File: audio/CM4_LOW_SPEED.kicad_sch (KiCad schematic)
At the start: 8 parts, among them J4 THD-02-R, U5 TPD4EUSB30, U6 TPD4EUSB30, U7 MagJack-A70-112-331N126

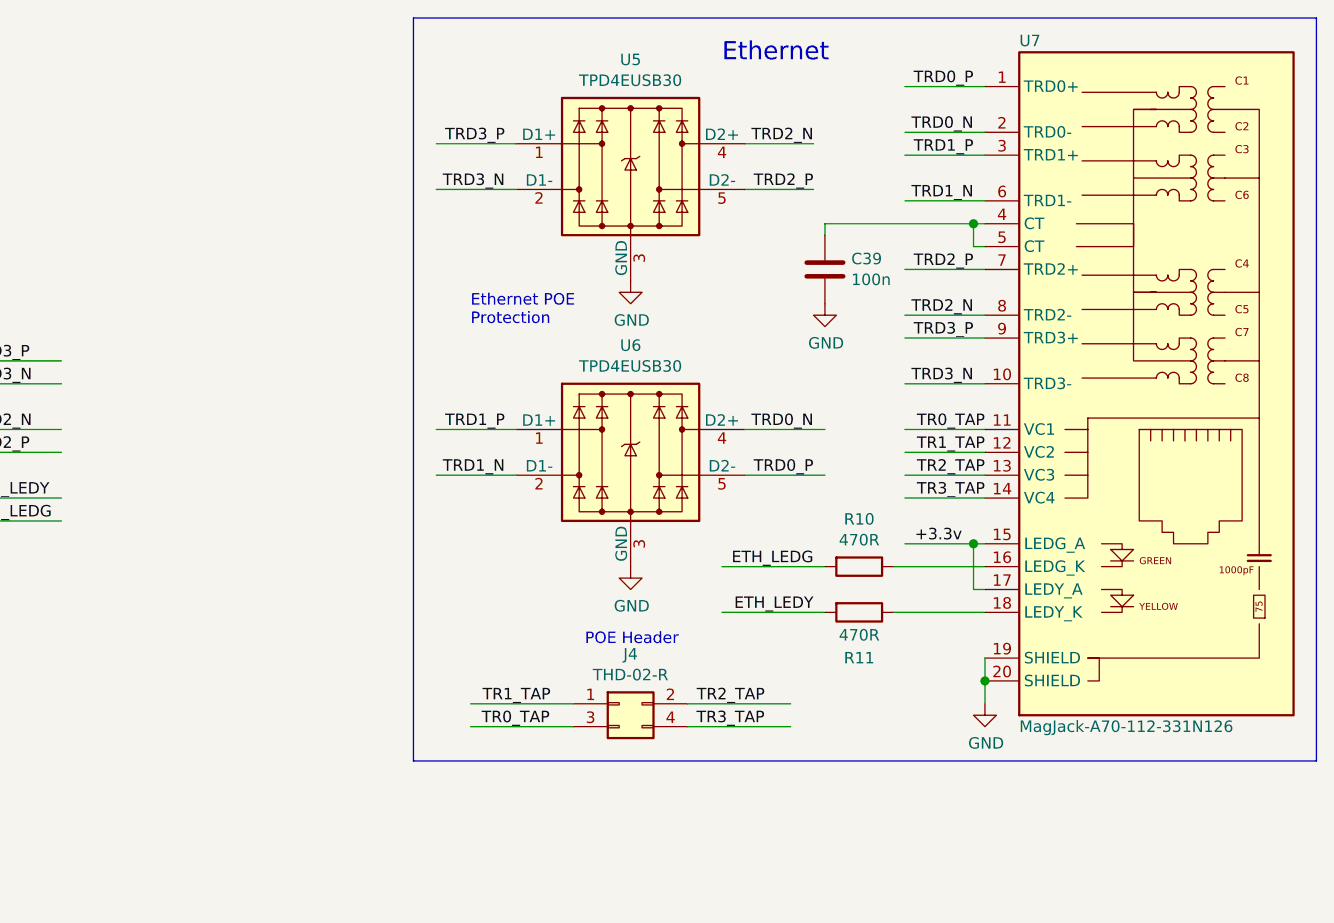
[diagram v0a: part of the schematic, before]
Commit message: .
.
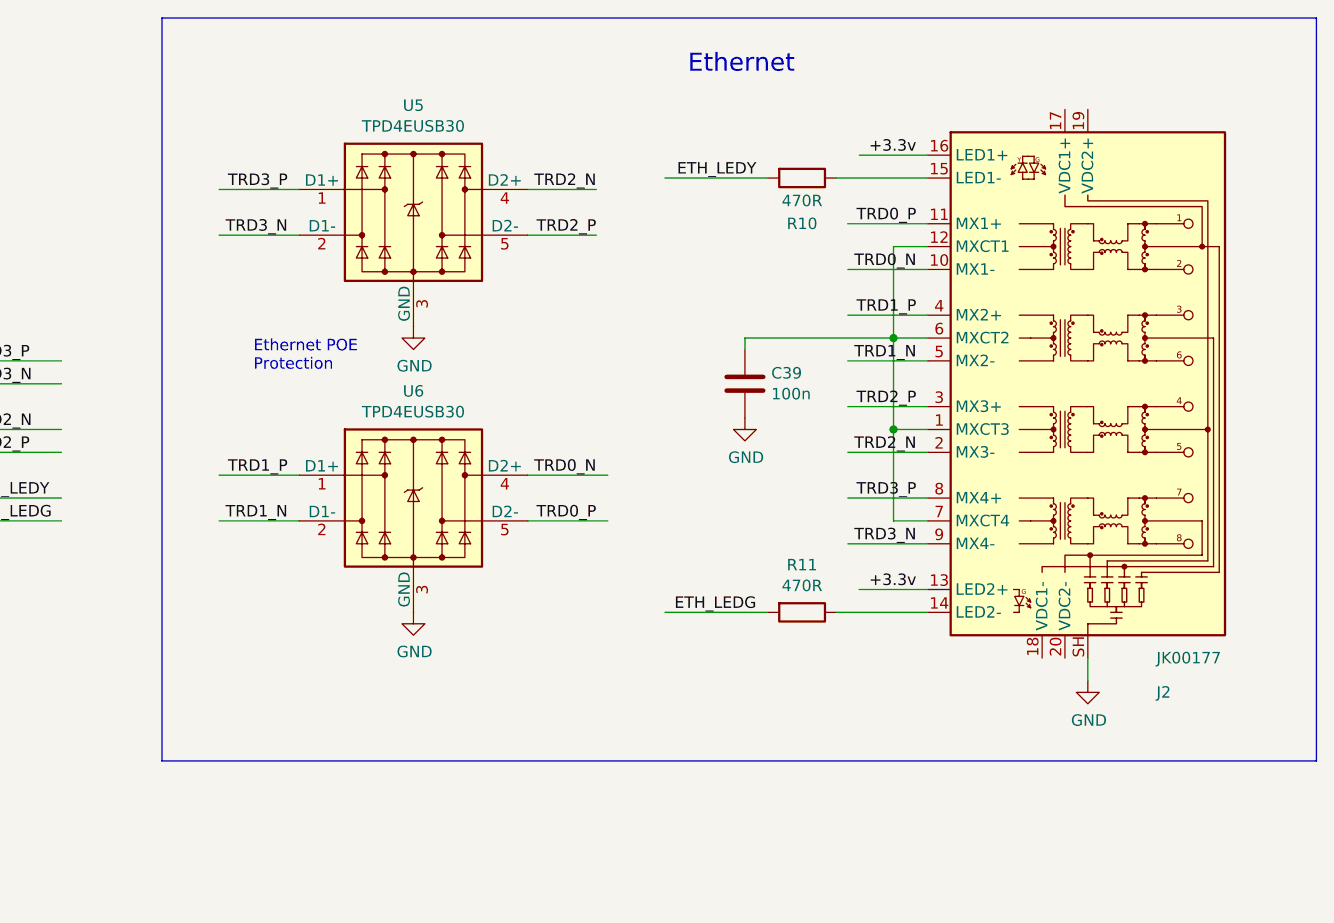
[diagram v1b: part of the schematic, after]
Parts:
- removed J4: THD-02-R, Connector_PinHeader_2.54mm:PinHeader_2x02_P2.54mm_Vertical, symbol Connector_Generic:Conn_02x02_Odd_Even
- removed U7: MagJack-A70-112-331N126, CM4IO:TRJG0926HENL, symbol CM4IO:MagJack-A70-112-331N126
- added J2: JK00177, Connector_RJ:RJ45_Pulse_JK00177NL_Horizontal, symbol Connector:JK00177
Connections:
- net +3.3v: now also J2.13 (LED2+), J2.16 (LED1+)
- net ETH_LEDG: now also R11.2; no longer R10.2
- net ETH_LEDY: now also R10.2; no longer R11.2
- net GND: now also J2.SH
- net TRD0_N: now also J2.10 (MX1-)
- net TRD0_P: now also J2.11 (MX1+)
- net TRD1_N: now also J2.5 (MX2-)
- net TRD1_P: now also J2.4 (MX2+)
- net TRD2_N: now also J2.2 (MX3-)
- net TRD2_P: now also J2.3 (MX3+)
- net TRD3_N: now also J2.9 (MX4-)
- net TRD3_P: now also J2.8 (MX4+)
- net at R10.1: now also J2.15 (LED1-)
- net at R11.1: now also J2.14 (LED2-)
- net at C39.1: now also J2.1 (MXCT3), J2.12 (MXCT1), J2.6 (MXCT2), J2.7 (MXCT4)
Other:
- note removed: "POE Header"
- moved on the sheet: U5, U6

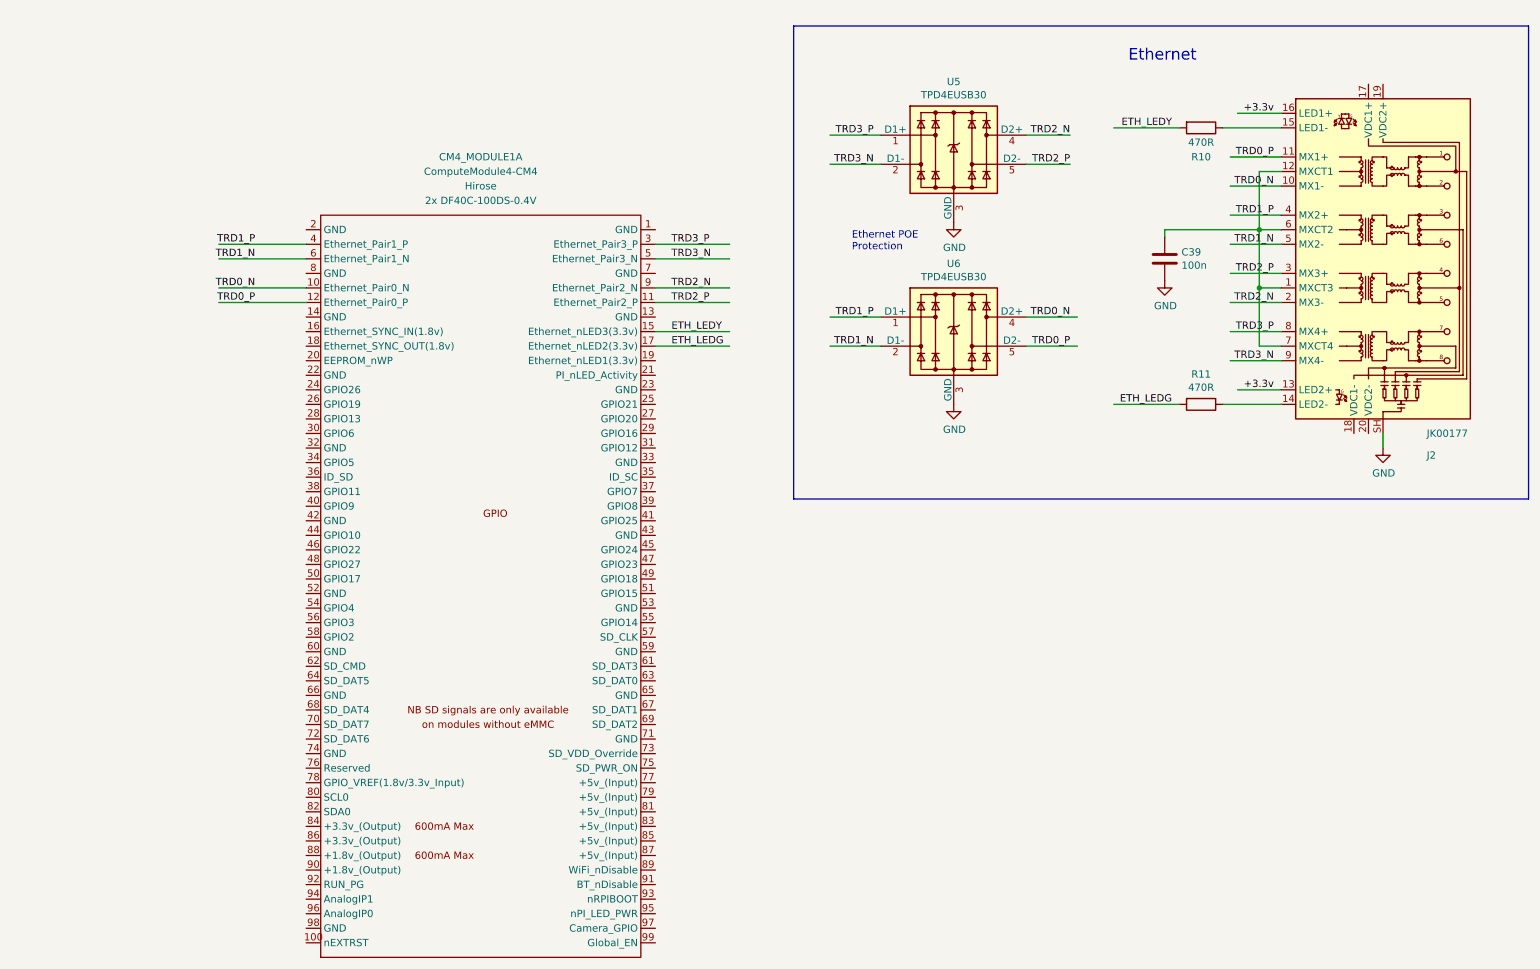
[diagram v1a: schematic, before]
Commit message: .
.
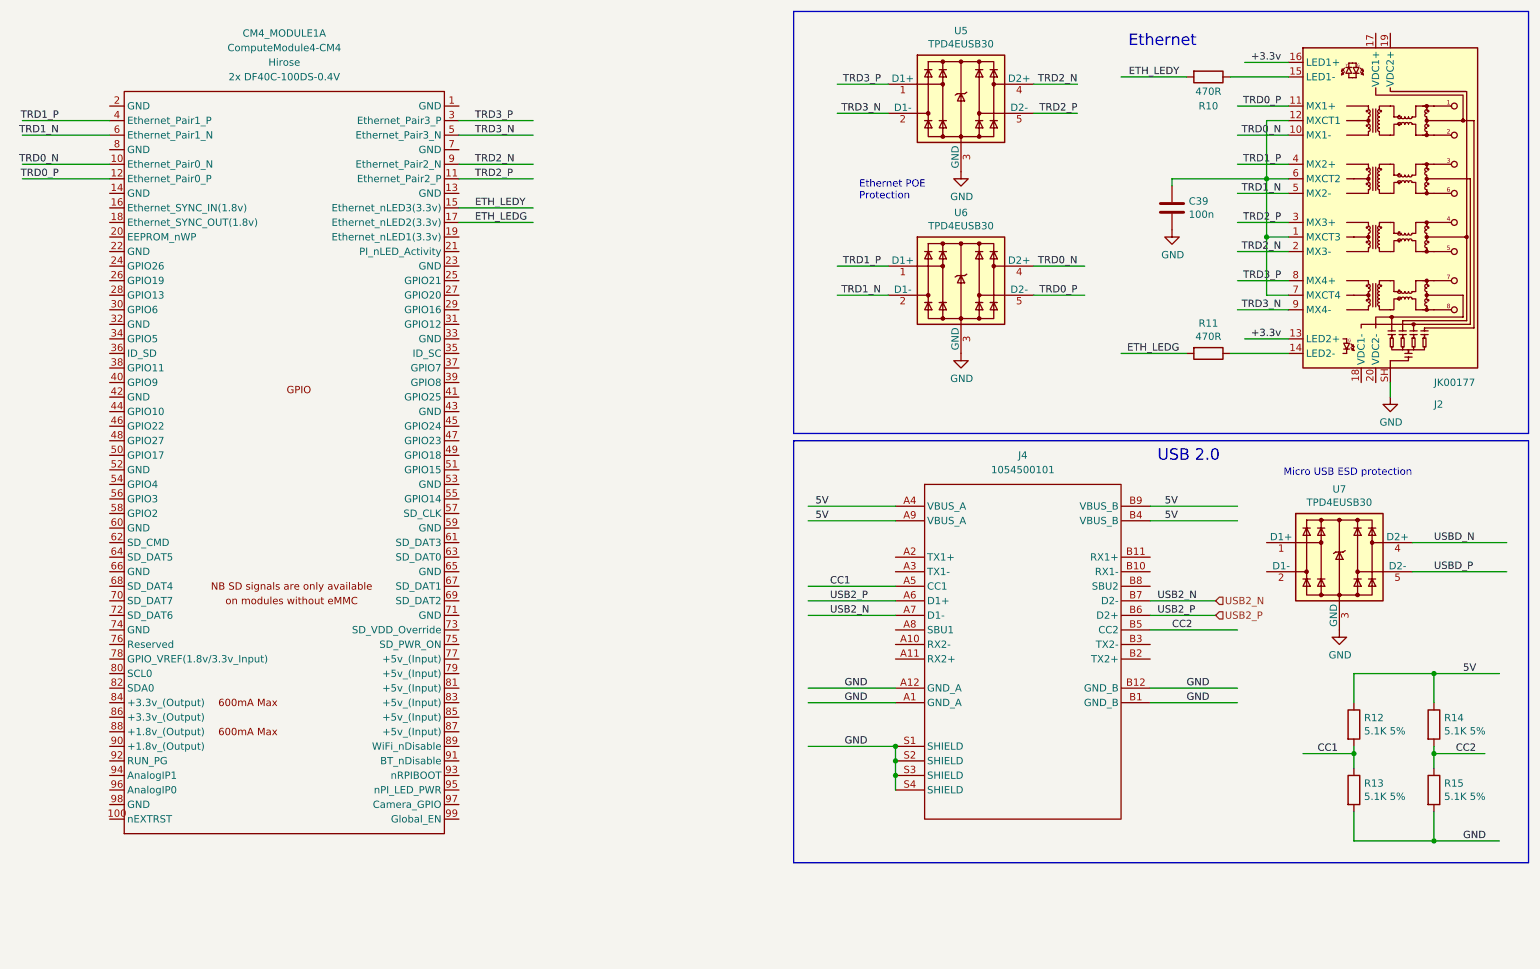
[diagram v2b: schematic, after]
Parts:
- added J4: 1054500101, CM4IO:MOLEX_105450-0101, symbol CM4IO:1054500101
- added R12, R13, R14, R15: 5.1K 5%, Resistor_SMD:R_0402_1005Metric, symbol Device:R
- added U7: TPD4EUSB30, Package_SON:USON-10_2.5x1.0mm_P0.5mm, symbol CM4IO:TPD4EUSB30
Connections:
- net GND: now also J4.A1 (GND_A), J4.A12 (GND_A), J4.B1 (GND_B), J4.B12 (GND_B), J4.S1 (SHIELD), J4.S2 (SHIELD), J4.S3 (SHIELD), J4.S4 (SHIELD), R13.2, R15.2, U7.3 (GND), U7.8 (GND)
- new net: U7.1 (D1+), U7.10
- new net: U7.2 (D1-), U7.9
- new net 5V: J4.A4 (VBUS_A), J4.A9 (VBUS_A), J4.B4 (VBUS_B), J4.B9 (VBUS_B), R12.1, R14.1
- new net CC1: J4.A5 (CC1), R12.2, R13.1
- new net CC2: J4.B5 (CC2), R14.2, R15.1
- new net USB2_N: J4.A7 (D1-), J4.B7 (D2-)
- new net USB2_P: J4.A6 (D1+), J4.B6 (D2+)
- new net USBD_N: U7.4 (D2+), U7.7
- new net USBD_P: U7.5 (D2-), U7.6
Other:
- note added: "Micro USB ESD protection"
- note added: "USB 2.0"
- moved on the sheet: C39, CM4_MODULE1A, J2, R10, R11, U5, U6
